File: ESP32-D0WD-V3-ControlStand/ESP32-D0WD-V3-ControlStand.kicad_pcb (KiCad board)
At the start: 2 copper layers, 184.1 x 144.1 mm, 193 parts, among them J1 Button & LED Panel, J10 RJ45, J11 Barrel_Jack, J12 Battery, J13 USB_OTG, J2 Button & LED Panel, J3 STEMMA (Display), J4 Horn, J5 Brake, J6 Light Switch, J7 Reverser, J8 Throttle, J9 RJ45, P1 CONN_8, P2 Misc buttons, bell, status LED, P6 CONN_3, P7 CONN_3, P8 CONN_5, P9 CONN_5, Q1 UMH3N, SW1 A, SW10 SW_PUSH_SMALL, SW11 SW_PUSH_SMALL, SW12 SW_PUSH_SMALL, SW13 SW_PUSH_SMALL, SW14 SW_PUSH_SMALL, SW15 SW_PUSH_SMALL, SW16 SW_PUSH_SMALL, SW17 SW_PUSH_SMALL, SW18 SW_PUSH_SMALL, SW19 SW_PUSH_SMALL, SW2 B, SW20 SW_PUSH_SMALL, SW21 SW_PUSH_SMALL, SW22 SW_PUSH_SMALL, SW23 On/Off, SW24 RESET, SW3 C, SW4 D, SW5 Bell, SW7 SW_PUSH_SMALL, SW8 SW_PUSH_SMALL, SW9 SW_PUSH_SMALL, T1 Buttons, T2 LEDS, T3 Buttons, T4 LEDS, T5 + 15 in -, T6 + 15 out -, U1 MCP23017, U10 ESP32-D0WD-V3, U11 W25Q32JVSSIQ, U2 TBD62083A, U3 MCP23017, U4 TBD62083A, U5 TCAN332DR, U6 MCP73871, U7 LM2574HVM-5.0, U8 TC1263-3.3VOATR, U9 FT231XS-R, Y1 40 Mhz +/- 10 ppm

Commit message: Started on V0.1 PCB.
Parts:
- moved MK1 223.1 mm to (134.8, 228.4)
- moved MK13 221.6 mm to (134.8, 228.4)
- moved MK23 217.1 mm to (134.8, 228.4)
- moved SW5 216.1 mm to (134.8, 228.4), turned to 0 degrees
- moved MK9 215.9 mm to (134.8, 228.4)
- moved D17 214.0 mm to (134.8, 228.4)
- moved T3 213.0 mm to (134.8, 228.4), turned to 0 degrees
- moved MK2 210.4 mm to (134.8, 228.4)
- moved SW22 209.9 mm to (134.8, 228.4), turned to 0 degrees
- moved MK16 208.8 mm to (134.8, 228.4)
- moved MK10 208.2 mm to (134.8, 228.4)
- moved D16 206.9 mm to (134.8, 228.4)
- moved T1 206.6 mm to (134.8, 228.4), turned to 0 degrees
- moved MK24 204.9 mm to (134.8, 228.4)
- moved SW21 202.7 mm to (134.8, 228.4), turned to 0 degrees
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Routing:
- net GND: track 587.8 -> 32.4 mm, vias 64 -> 25
- net +BATT: track 285.1 -> 0.00 mm, vias 2 -> 0
- net +5V: track 195.4 -> 0.00 mm, vias 5 -> 0
- net +3V3: track 205.9 -> 34.0 mm, vias 15 -> 2
- net +12V: track 129.9 -> 0.00 mm, vias 4 -> 0
- net /L_Ditch: track 106.7 -> 1.20 mm, vias 7 -> 1
- net Net-(D17-Pad2): track 101.2 -> 0.00 mm, vias 3 -> 0
- net Net-(D2-Pad2): track 100.5 -> 0.00 mm, vias 3 -> 0
- net /CAN_RX: track 97.6 -> 0.48 mm, vias 6 -> 1
- net Net-(P1-Pad6): track 94.9 -> 0.00 mm, vias 4 -> 0
- net /CAN_TX: track 100.8 -> 6.65 mm, vias 4 -> 1
- net Net-(D3-Pad2): track 88.9 -> 0.00 mm, vias 3 -> 0
- net Net-(D16-Pad2): track 88.9 -> 0.00 mm, vias 3 -> 0
- net Net-(SW7-Pad1): track 87.6 -> 0.00 mm, vias 3 -> 0
- net Net-(D4-Pad2): track 86.3 -> 0.00 mm, vias 3 -> 0
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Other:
- board outline removed
- rule pad_to_mask_clearance: 0.2 -> 0
- board text removed: "Adafruit 1.3" 128x64 STEMMA OLED"

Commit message: About halfway done.
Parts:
- moved T6 161.7 mm to (242.6, 108.0), turned to 90 degrees
- moved D19 157.7 mm to (242.6, 113.3), turned to 90 degrees
- moved J9 141.9 mm to (207.6, 106.7), turned to 180 degrees
- moved L1 141.5 mm to (227.5, 121.5)
- moved D27 140.9 mm to (238.6, 133.2), turned to 90 degrees
- moved P7 139.5 mm to (54.6, 114.3), turned to 180 degrees
- moved D18 139.0 mm to (242.6, 140.7), turned to 90 degrees
- moved MK7 135.8 mm to (78.7, 104.8)
- moved EN2 135.4 mm to (67.3, 111.0), turned to 270 degrees
- moved U7 134.7 mm to (230.4, 133.6), turned to 90 degrees
- moved T5 134.1 mm to (242.6, 148.6), turned to 90 degrees
- moved MK19 130.3 mm to (174.0, 104.1)
- moved C5 130.1 mm to (194.1, 112.6), turned to 90 degrees
- moved MK5 129.3 mm to (54.6, 127.0)
- moved C8 127.8 mm to (230.6, 143.9)
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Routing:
- net +5V: track 0.00 -> 253.8 mm, vias 0 -> 16
- net GND: track 32.4 -> 207.5 mm, vias 25 -> 49
- net +12V: track 0.00 -> 99.1 mm, vias 0 -> 5
- net /Button_A: track 4.30 -> 67.7 mm, vias 0 -> 3
- net /CAN Transceiver/CANH: track 0.00 -> 52.4 mm, vias 0 -> 3
- net /Processor Section/RX: track 0.00 -> 47.1 mm, vias 0 -> 6
- net Net-(C6-Pad1): track 0.00 -> 46.7 mm, vias 0 -> 4
- net /CAN_TX: track 6.65 -> 53.2 mm, vias 1 -> 4
- net /CAN Transceiver/CANL: track 0.00 -> 45.9 mm, vias 0 -> 3
- net Net-(C9-Pad1): track 0.00 -> 42.1 mm, vias 0 -> 4
- net /CAN_RX: track 0.48 -> 41.8 mm, vias 1 -> 2
- net /L_Dim: track 2.70 -> 43.8 mm, vias 1 -> 4
- net /SDA: track 5.83 -> 46.7 mm, vias 0 -> 1
- net VBUS: track 0.00 -> 38.4 mm, vias 0 -> 5
- net /SCL: track 4.77 -> 41.8 mm, vias 0 -> 1
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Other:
- board outline added: 198.1 x 54 mm

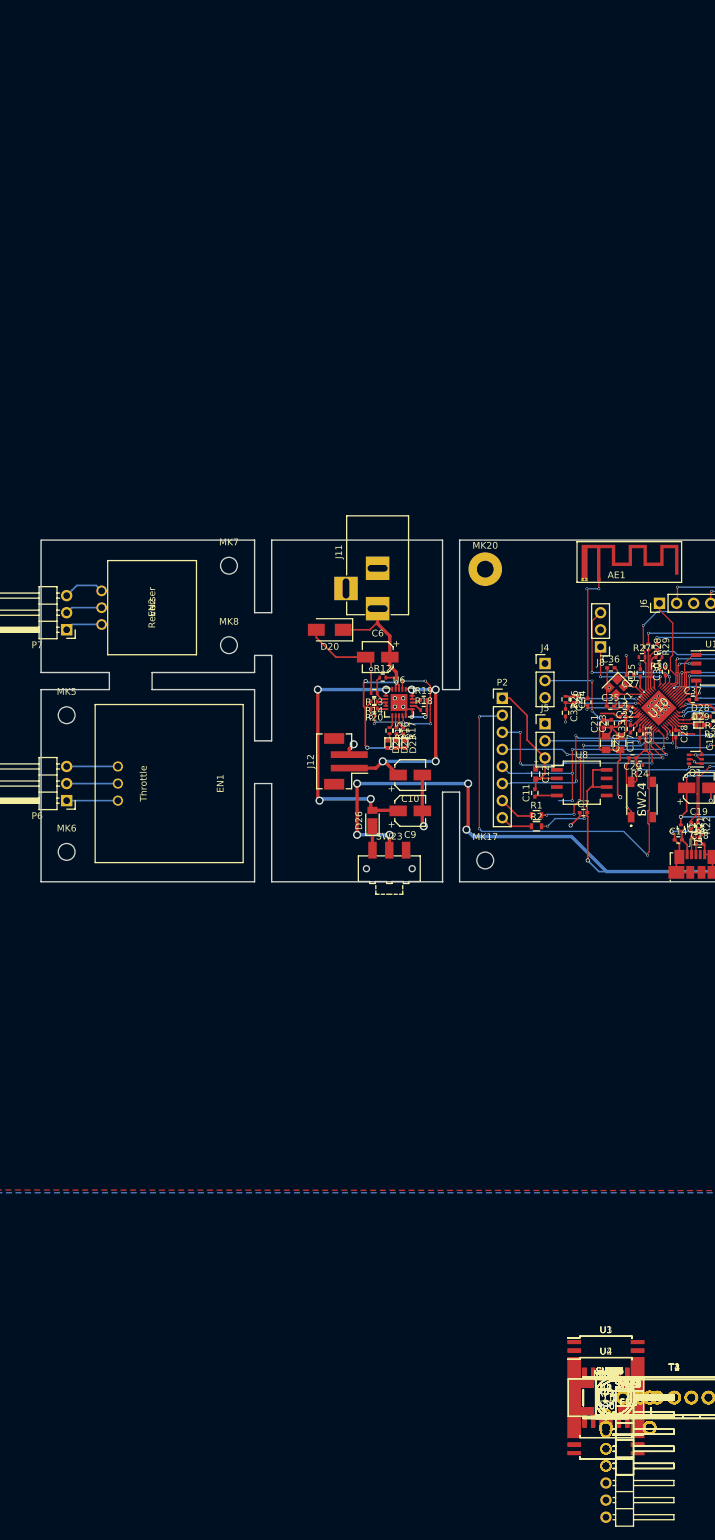
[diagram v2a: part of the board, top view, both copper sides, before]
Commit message: Nearly done.  Just the button/LED boards to do.
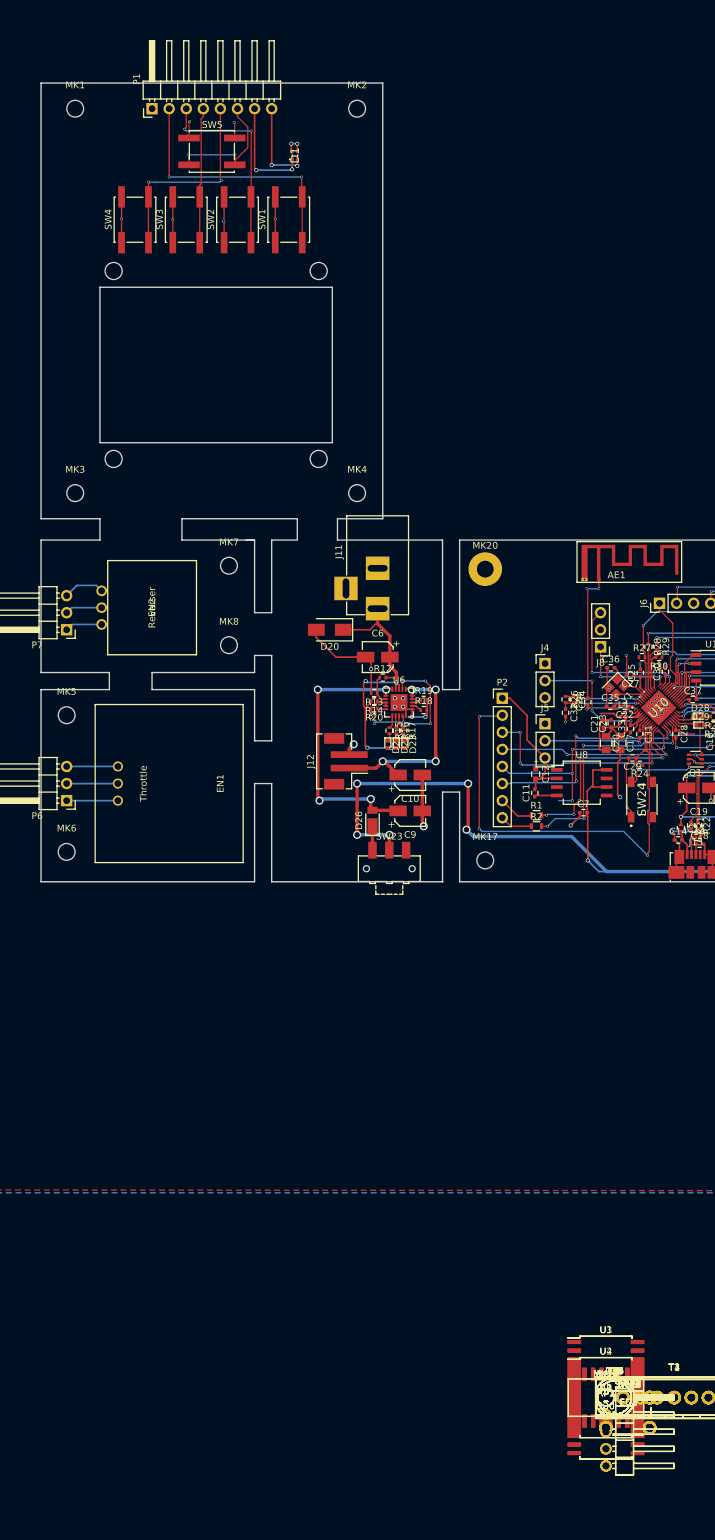
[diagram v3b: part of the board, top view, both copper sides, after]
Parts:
- added REF**: 128x64OLEDSTEMMA, AdafruitDisplays:128x64OLEDSTEMMA, F.Cu at (76.8, 77.5)
- moved MK1 207.2 mm to (55.9, 36.8)
- moved P1 203.2 mm to (67.3, 36.8), turned to 90 degrees
- moved MK2 195.2 mm to (97.8, 36.8)
- moved SW5 194.3 mm to (76.2, 43.2)
- moved D1 190.4 mm to (88.5, 43.8), turned to 270 degrees
- moved SW4 188.6 mm to (64.8, 53.3), turned to 90 degrees
- moved SW3 185.9 mm to (72.4, 53.3), turned to 90 degrees
- moved SW2 183.5 mm to (80.0, 53.3), turned to 90 degrees
- moved SW1 181.3 mm to (87.6, 53.3), turned to 90 degrees
- moved MK3 155.9 mm to (55.9, 94.0)
- moved MK4 139.5 mm to (97.8, 94.0)
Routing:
- net Net-(P1-Pad2): track 0.00 -> 39.6 mm, vias 0 -> 2
- net GND: track 207.5 -> 242.8 mm, vias 49 -> 58
- net Net-(P1-Pad5): track 0.00 -> 30.6 mm, vias 0 -> 2
- net Net-(P1-Pad3): track 0.00 -> 29.8 mm, vias 0 -> 2
- net Net-(P1-Pad4): track 0.00 -> 20.1 mm
- net Net-(P1-Pad6): track 0.00 -> 19.7 mm, vias 0 -> 2
- net Net-(D1-Pad1): track 0.00 -> 16.1 mm, vias 0 -> 2
- net Net-(D1-Pad3): track 0.00 -> 13.2 mm, vias 0 -> 2
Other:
- board size 198.1 x 54 mm -> 198.1 x 121.9 mm
